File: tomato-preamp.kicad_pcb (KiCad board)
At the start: 2 copper layers, 77 x 69.8 mm, 23 parts, among them J1 IN, J2 OUT, J3.1 +ANODE, J3.2 -ANODE, J4.1 +HEATER, J4.2 -HEATER, U1 6N2P

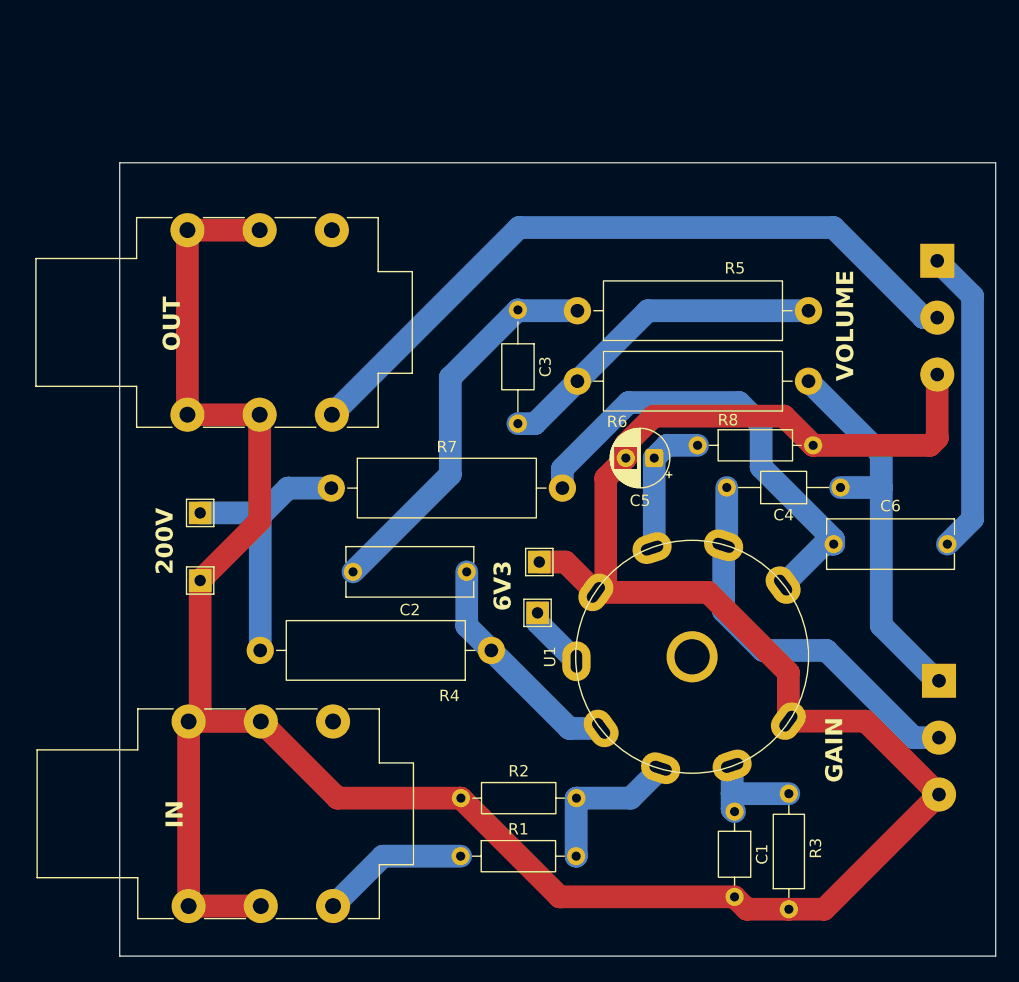
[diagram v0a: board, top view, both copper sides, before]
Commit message: Rewire
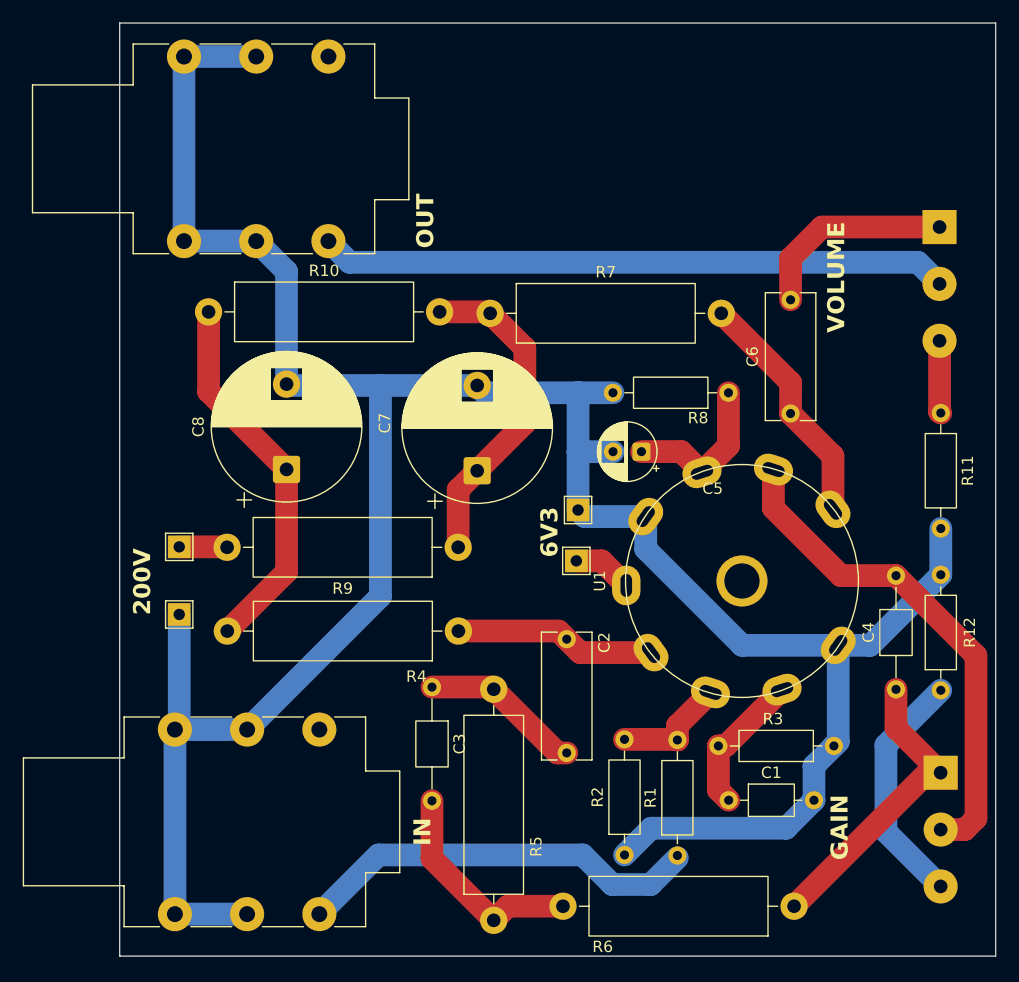
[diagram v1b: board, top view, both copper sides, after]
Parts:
- added C7: 22u 400V, Capacitor_THT:CP_Radial_D13.0mm_P7.50mm, F.Cu at (131.4, 89.4)
- added C8: 22u 400V, Capacitor_THT:CP_Radial_D13.0mm_P7.50mm, F.Cu at (114.7, 89.3)
- added R10: 1K 2W, Resistor_THT:R_Axial_DIN0516_L15.5mm_D5.0mm_P20.32mm_Horizontal, F.Cu at (107.8, 75.4)
- added R11: 1K, Resistor_THT:R_Axial_DIN0207_L6.3mm_D2.5mm_P10.16mm_Horizontal, F.Cu at (172.2, 84.3)
- added R12: 1K, Resistor_THT:R_Axial_DIN0207_L6.3mm_D2.5mm_P10.16mm_Horizontal, F.Cu at (172.2, 108.7)
- added R9: 1K 2W, Resistor_THT:R_Axial_DIN0516_L15.5mm_D5.0mm_P20.32mm_Horizontal, F.Cu at (129.8, 96.1)
- R4, R7: value 32k -> 32k 2W
- moved R5 60.3 mm to (132.9, 128.9), turned to 90 degrees
- moved R6 46.2 mm to (159.3, 127.7)
- moved C3 34.0 mm to (127.5, 108.4)
- moved R7 20.8 mm to (132.6, 75.6)
- moved R1 19.1 mm to (149.1, 123.2), turned to 90 degrees
- moved C4 18.4 mm to (168.3, 108.6), turned to 90 degrees
- moved J2 15.3 mm to (118.4, 69.2)
- moved R2 15.2 mm to (144.4, 123.2), turned to 90 degrees
- moved R3 14.9 mm to (162.8, 113.6), turned to 180 degrees
- moved C6 12.1 mm to (159.0, 84.4), turned to 90 degrees
- moved C2 10.6 mm to (139.3, 104.2), turned to -90 degrees
- moved RV1 8.08 mm to (172.2, 116.0)
- moved U1 7.98 mm to (162.7, 92.8)
- moved J4.1 5.70 mm to (140.2, 97.3)
- moved J4.2 5.70 mm to (140.3, 92.9)
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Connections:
- J3.1 pad 1: /High voltage -> Net-(J3.1-Pin_1)
- R4 pad 2: /High voltage -> Net-(C8-Pad1)
- R7 pad 1: /High voltage -> Net-(C7-Pad1)
- RV1 pad 3: GND -> Net-(R12-Pad1)
- RV2 pad 3: GND -> Net-(R11-Pad1)
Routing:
- net Net-(C8-Pad1): track 0.00 -> 33.1 mm
- net Net-(C7-Pad1): track 0.00 -> 28.8 mm
- net /High voltage: track 24.4 -> 0.00 mm
- net Net-(J1-PadT): track 13.0 -> 35.7 mm
- net Net-(R12-Pad1): track 0.00 -> 21.2 mm
- net Net-(U1B-A): track 41.5 -> 21.3 mm
- net Net-(C2-Pad2): track 34.3 -> 14.2 mm
- net GND: track 253.7 -> 237.6 mm
- net Net-(C3-Pad2): track 29.7 -> 19.4 mm
- net Net-(U1B-G): track 34.3 -> 44.4 mm
- net Net-(C6-Pad2): track 27.1 -> 17.9 mm
- net Net-(J2-PadT): track 63.3 -> 55.3 mm
- net Net-(C4-Pad1): track 34.6 -> 26.7 mm
- net Net-(R11-Pad1): track 0.00 -> 6.39 mm
- net Net-(J3.1-Pin_1): track 0.00 -> 4.22 mm
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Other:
- board size 77 x 69.8 mm -> 77 x 82 mm
